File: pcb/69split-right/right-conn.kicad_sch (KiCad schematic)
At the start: 1 part, among them J3 USB_C_Receptacle

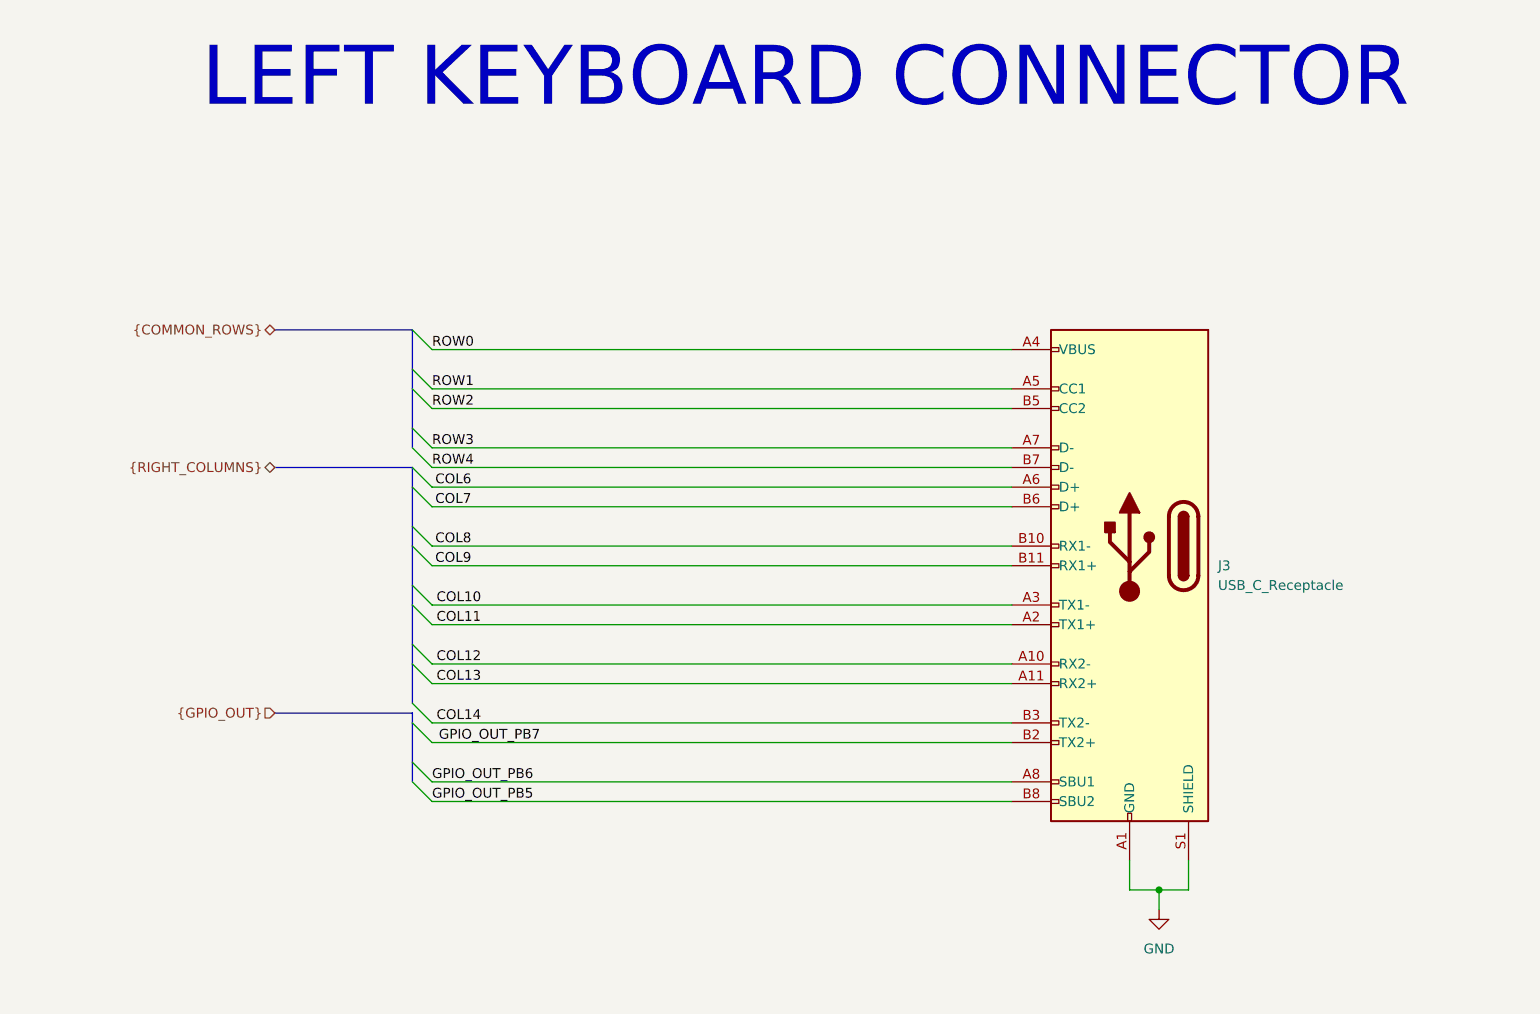
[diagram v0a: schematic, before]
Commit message: Moved things around so it's less confusing.
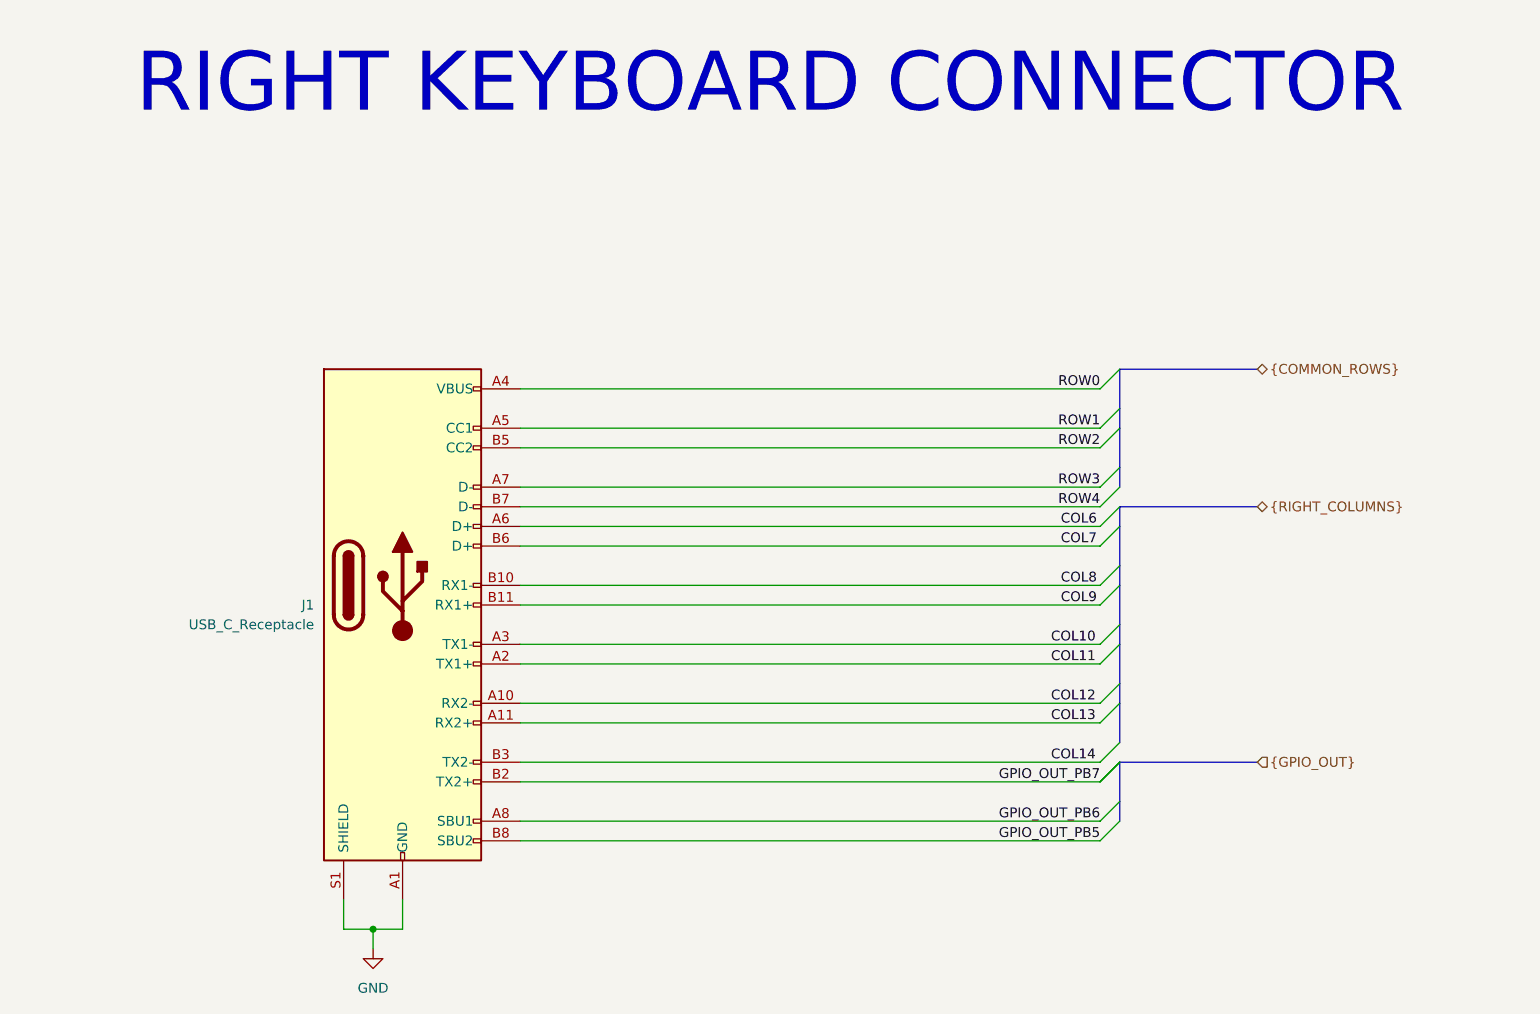
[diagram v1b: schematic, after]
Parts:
- removed J3: USB_C_Receptacle, Connector_USB:USB_C_Receptacle_Amphenol_12401548E4-2A, symbol Connector:USB_C_Receptacle
- added J1: USB_C_Receptacle, Connector_USB:USB_C_Receptacle_Amphenol_12401548E4-2A, symbol Connector:USB_C_Receptacle
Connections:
- net COL10: now also J1.A3 (TX1-)
- net COL11: now also J1.A2 (TX1+)
- net COL12: now also J1.A10 (RX2-)
- net COL13: now also J1.A11 (RX2+)
- net COL14: now also J1.B3 (TX2-)
- net COL6: now also J1.A6 (D+)
- net COL7: now also J1.B6 (D+)
- net COL8: now also J1.B10 (RX1-)
- net COL9: now also J1.B11 (RX1+)
- net GND: now also J1.A1 (GND), J1.A12 (GND), J1.B1 (GND), J1.B12 (GND), J1.S1 (SHIELD)
- net GPIO_OUT_PB5: now also J1.B8 (SBU2)
- net GPIO_OUT_PB6: now also J1.A8 (SBU1)
- net GPIO_OUT_PB7: now also J1.B2 (TX2+)
- net ROW0: now also J1.A4 (VBUS), J1.A9 (VBUS), J1.B4 (VBUS), J1.B9 (VBUS)
- net ROW1: now also J1.A5 (CC1)
- net ROW2: now also J1.B5 (CC2)
- net ROW3: now also J1.A7 (D-)
- net ROW4: now also J1.B7 (D-)
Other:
- note added: "RIGHT KEYBOARD CONNECTOR"
- note removed: "LEFT KEYBOARD CONNECTOR"
